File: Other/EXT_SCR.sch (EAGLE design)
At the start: 15 parts, among them IC1 MCP23016-I/SO

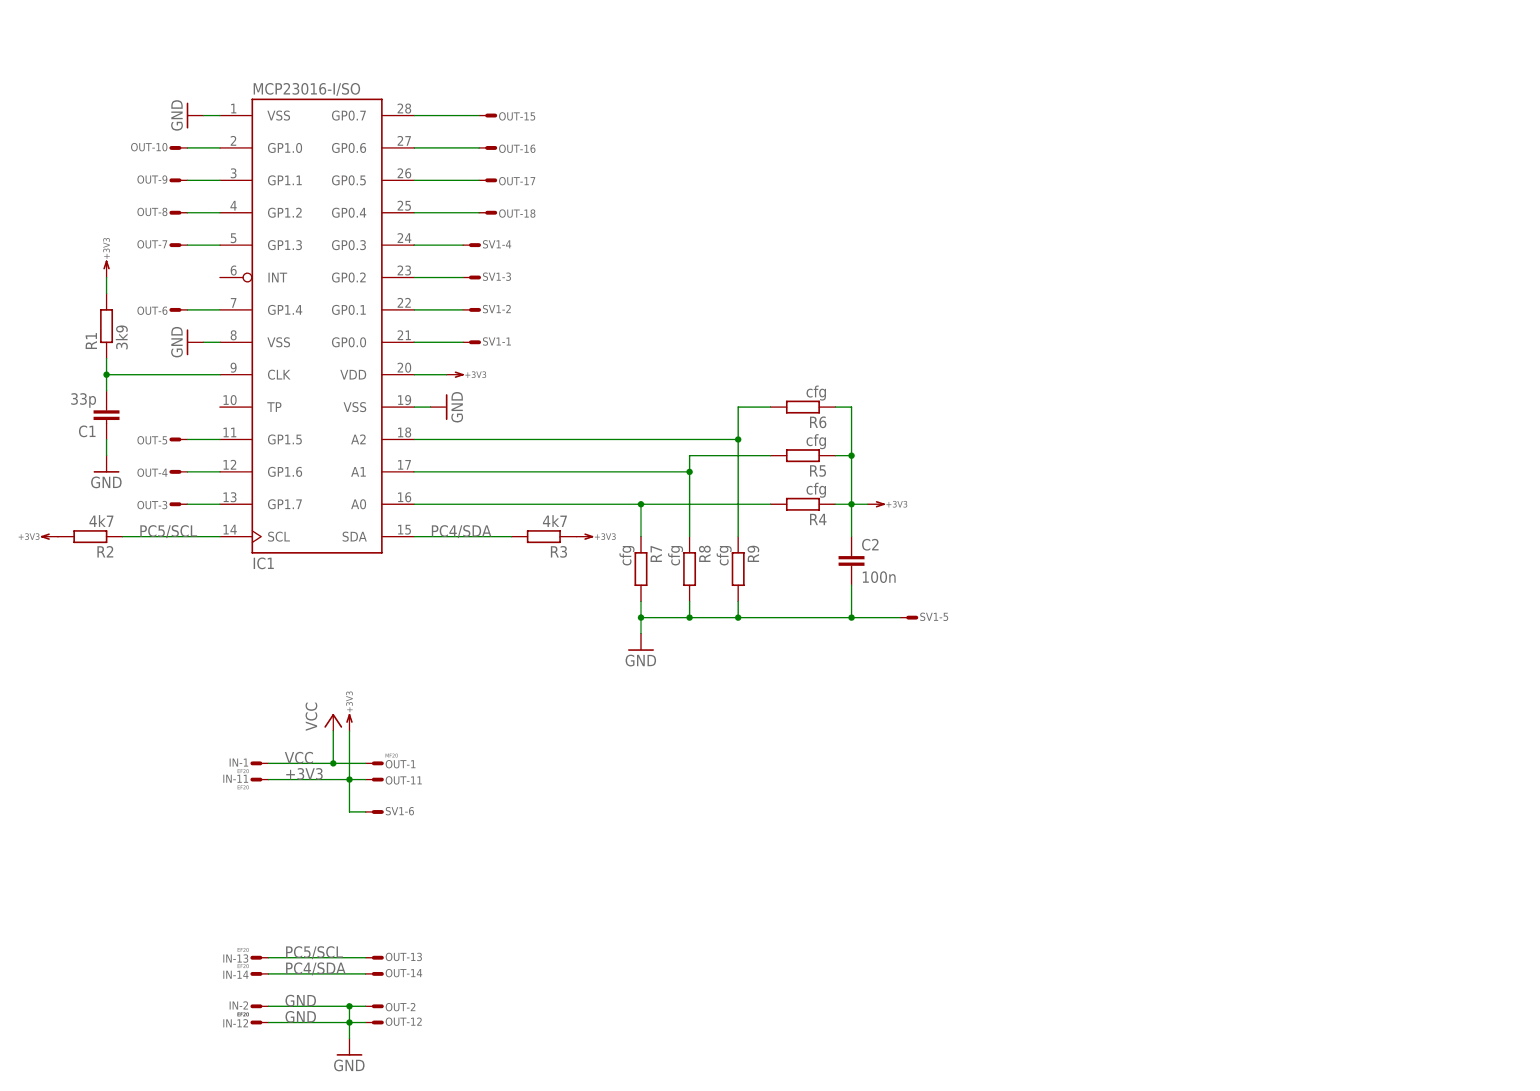
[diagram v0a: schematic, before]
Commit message: Added ...
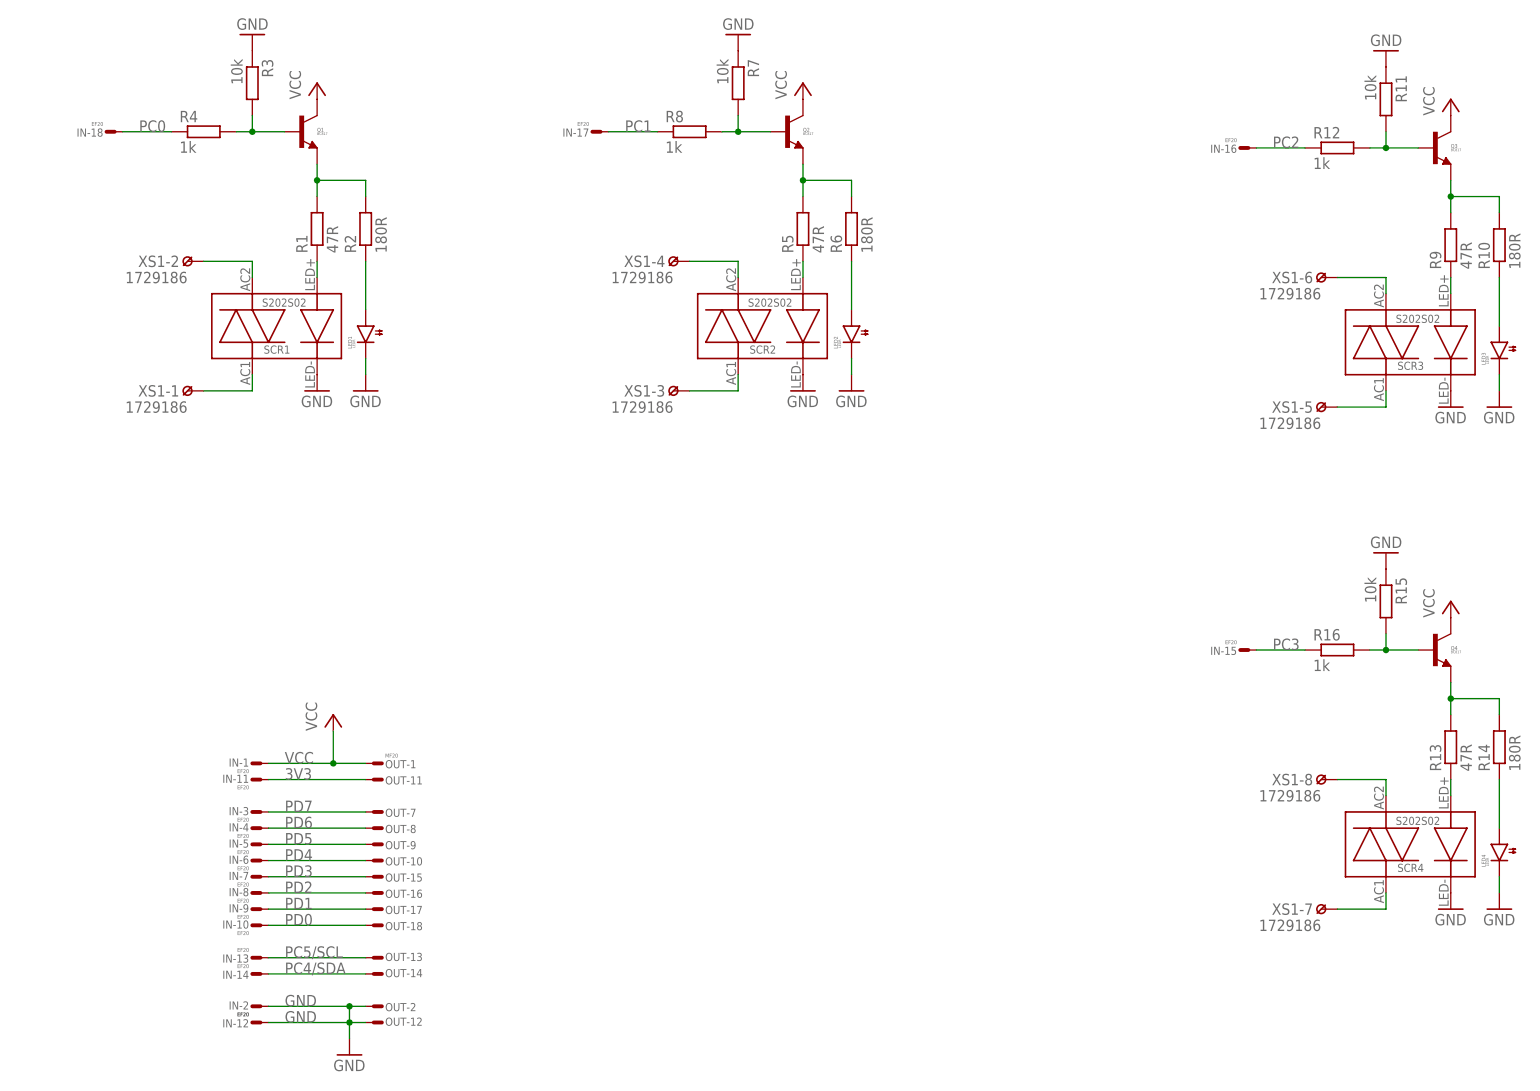
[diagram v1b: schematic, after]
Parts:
- removed C1: 33p, RCL:C0603
- removed C2: 100n, RCL:C0603
- removed IC1: MCP23016-I/SO, ICs:MCP23016-I/SO
- removed SV1: (no value), Conn:ML6ES
- added LED1, LED2, LED3, LED4: LEDR, Optic:LED1206
- added Q1, Q2, Q3, Q4: BC817, Transistor:NPN23
- added R10, R14: 180R, RCL:R0603
- added R11, R15: 10k, RCL:R0603
- added R12, R16: 1k, RCL:R0603
- added R13: 47R, RCL:R0603
- added SCR1, SCR2, SCR3, SCR4: S202S02, Relay_Switch:S202
- added XS1: 1729186, Conn:CON8-SS508
- IN: device Conn:FE20ELSS -> Conn:FE20ELS
- R1: value 3k9 -> 47R
- R2: value 4k7 -> 180R
- R3: value 4k7 -> 10k
- R4, R8: value cfg -> 1k
- R5, R9: value cfg -> 47R
- R6: value cfg -> 180R
- R7: value cfg -> 10k
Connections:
- removed net +3V3: C2.1, IC1.VDD, IN-11.S, OUT-11.S, R1.2, R2.2, R3.1, R4.1, R5.1, R6.1, SV1-6.S
- new net 3V3: IN-11.S, OUT-11.S
- new net N$21: SCR3.AC1, XS1-5.K
- new net N$22: SCR3.AC2, XS1-6.K
- new net N$23: SCR4.AC2, XS1-8.K
- new net N$24: SCR4.AC1, XS1-7.K
- new net PC0: IN-18.S, R4.1
- new net PC1: IN-17.S, R8.1
- new net PC2: IN-16.S, R12.1
- new net PC3: IN-15.S, R16.1
- new net PD0: IN-10.S, OUT-18.S
- new net PD1: IN-9.S, OUT-17.S
- new net PD2: IN-8.S, OUT-16.S
- new net PD3: IN-7.S, OUT-15.S
- new net PD4: IN-6.S, OUT-10.S
- new net PD5: IN-5.S, OUT-9.S
- new net PD6: IN-4.S, OUT-8.S
- new net PD7: IN-3.S, OUT-7.S
- net GND: now also LED1.C, LED2.C, LED3.C, LED4.C, R11.1, R15.1, R3.1, R7.1, SCR1.L-, SCR2.L-, SCR3.L-, SCR4.L-; no longer C1.1, C2.2, IC1.VSS@1, IC1.VSS@19, IC1.VSS@8, R7.2, R8.2, R9.2, SV1-5.S
- net N$1: now also SCR1.L+; no longer C1.2, IC1.CLK
- net N$10: now also LED3.A, R10.1; no longer IC1.A0, R4.2, R7.1
- net N$11: now also Q3.E, R10.2, R9.2; no longer IC1.A1, R5.2, R8.1
- net N$12: now also Q3.B, R11.2, R12.2; no longer IC1.A2, R6.2, R9.1
- net N$13: now also R13.1, SCR4.L+; no longer IC1.GP0.0, SV1-1.S
- net N$14: now also LED4.A, R14.1; no longer IC1.GP0.1, SV1-2.S
- net N$15: now also Q4.E, R13.2, R14.2; no longer IC1.GP0.2, SV1-3.S
- net N$16: now also Q4.B, R15.2, R16.2; no longer IC1.GP0.3, SV1-4.S
- net N$17: now also SCR1.AC1, XS1-1.K; no longer IC1.GP0.4, OUT-18.S
- net N$18: now also SCR1.AC2, XS1-2.K; no longer IC1.GP0.5, OUT-17.S
- net N$19: now also SCR2.AC1, XS1-3.K; no longer IC1.GP0.6, OUT-16.S
- net N$2: now also LED1.A, R2.1; no longer IC1.GP1.4, OUT-6.S
- net N$20: now also SCR2.AC2, XS1-4.K; no longer IC1.GP0.7, OUT-15.S
- net N$3: now also Q1.E, R1.2, R2.2; no longer IC1.GP1.3, OUT-7.S
- net N$4: now also Q1.B, R3.2, R4.2; no longer IC1.GP1.2, OUT-8.S
- net N$5: now also R5.1, SCR2.L+; no longer IC1.GP1.1, OUT-9.S
- net N$6: now also LED2.A, R6.1; no longer IC1.GP1.0, OUT-10.S
- net N$7: now also Q2.E, R5.2, R6.2; no longer IC1.GP1.5, OUT-5.S
- net N$8: now also Q2.B, R7.2, R8.2; no longer IC1.GP1.6, OUT-4.S
- net N$9: now also R9.1, SCR3.L+; no longer IC1.GP1.7, OUT-3.S
- net PC4/SDA: no longer IC1.SDA, R3.2
- net PC5/SCL: no longer IC1.SCL, R2.1
- net VCC: now also Q1.C, Q2.C, Q3.C, Q4.C
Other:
- moved on the sheet: OUT-10, OUT-15, OUT-16, OUT-17, OUT-18, OUT-7, OUT-8, OUT-9, R1, R2, R3, R4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

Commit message: Reorganization
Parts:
- IN: device Conn:FE20ELS -> Conn:FE20ELSS
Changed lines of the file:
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@@
 <?xml version="1.0" encoding="utf-8"?>
 <!DOCTYPE eagle SYSTEM "eagle.dtd">
-<eagle version="6.4">
+<eagle version="6.5.0">
 <drawing>
 <settings>
@@
 <grid distance="0.1" unitdist="inch" unit="inch" style="lines" multiple="1" display="no" altdistance="0.01" altunitdist="inch" altunit="inch"/>
 <layers>
-<layer number="1" name="Top" color="4" fill="1" visible="no" active="no"/>
-<layer number="2" name="Route2" color="1" fill="3" visible="no" active="no"/>
-<layer number="3" name="Route3" color="4" fill="3" visible="no" active="no"/>
-<layer number="4" name="Route4" color="1" fill="4" visible="no" active="no"/>
-<layer number="5" name="Route5" color="4" fill="4" visible="no" active="no"/>
-<layer number="6" name="Route6" color="1" fill="8" visible="no" active="no"/>
-<layer number="7" name="Route7" color="4" fill="8" visible="no" active="no"/>
-<layer number="8" name="Route8" color="1" fill="2" visible="no" active="no"/>
-<layer number="9" name="Route9" color="4" fill="2" visible="no" active="no"/>
-<layer number="10" name="Route10" color="1" fill="7" visible="no" active="no"/>
-<layer number="11" name="Route11" color="4" fill="7" visible="no" active="no"/>
-<layer number="12" name="Route12" color="1" fill="5" visible="no" active="no"/>
-<layer number="13" name="Route13" color="4" fill="5" visible="no" active="no"/>
-<layer number="14" name="Route14" color="1" fill="6" visible="no" active="no"/>
-<layer number="15" name="Route15" color="4" fill="6" visible="no" active="no"/>
-<layer number="16" name="Bottom" color="1" fill="1" visible="no" active="no"/>
-<layer number="17" name="Pads" color="2" fill="1" visible="no" active="no"/>
-<layer number="18" name="Vias" color="2" fill="1" visible="no" active="no"/>
-<layer number="19" name="Unrouted" color="6" fill="1" visible="no" active="no"/>
-<layer number="20" name="Dimension" color="15" fill="1" visible="no" active="no"/>
-<layer number="21" name="tPlace" color="7" fill="1" visible="no" active="no"/>
-<layer number="22" name="bPlace" color="7" fill="1" visible="no" active="no"/>
-<layer number="23" name="tOrigins" color="15" fill="1" visible="no" active="no"/>
-<layer number="24" name="bOrigins" color="15" fill="1" visible="no" active="no"/>
-<layer number="25" name="tNames" color="7" fill="1" visible="no" active="no"/>
-<layer number="26" name="bNames" color="7" fill="1" visible="no" active="no"/>
-<layer number="27" name="tValues" color="7" fill="1" visible="no" active="no"/>
-<layer number="28" name="bValues" color="7" fill="1" visible="no" active="no"/>
+<layer number="1" name="Top" color="4" fill="1" visible="yes" active="no"/>
+<layer number="2" name="Route2" color="1" fill="3" visible="yes" active="no"/>
+<layer number="3" name="Route3" color="4" fill="3" visible="yes" active="no"/>
+<layer number="4" name="Route4" color="1" fill="4" visible="yes" active="no"/>
+<layer number="5" name="Route5" color="4" fill="4" visible="yes" active="no"/>
+<layer number="6" name="Route6" color="1" fill="8" visible="yes" active="no"/>
+<layer number="7" name="Route7" color="4" fill="8" visible="yes" active="no"/>
+<layer number="8" name="Route8" color="1" fill="2" visible="yes" active="no"/>
+<layer number="9" name="Route9" color="4" fill="2" visible="yes" active="no"/>
+<layer number="10" name="Route10" color="1" fill="7" visible="yes" active="no"/>
+<layer number="11" name="Route11" color="4" fill="7" visible="yes" active="no"/>
+<layer number="12" name="Route12" color="1" fill="5" visible="yes" active="no"/>
+<layer number="13" name="Route13" color="4" fill="5" visible="yes" active="no"/>
+<layer number="14" name="Route14" color="1" fill="6" visible="yes" active="no"/>
+<layer number="15" name="Route15" color="4" fill="6" visible="yes" active="no"/>
+<layer number="16" name="Bottom" color="1" fill="1" visible="yes" active="no"/>
+<layer number="17" name="Pads" color="2" fill="1" visible="yes" active="no"/>
+<layer number="18" name="Vias" color="2" fill="1" visible="yes" active="no"/>
+<layer number="19" name="Unrouted" color="6" fill="1" visible="yes" active="no"/>
+<layer number="20" name="Dimension" color="15" fill="1" visible="yes" active="no"/>
+<layer number="21" name="tPlace" color="7" fill="1" visible="yes" active="no"/>
+<layer number="22" name="bPlace" color="7" fill="1" visible="yes" active="no"/>
+<layer number="23" name="tOrigins" color="15" fill="1" visible="yes" active="no"/>
+<layer number="24" name="bOrigins" color="15" fill="1" visible="yes" active="no"/>
+<layer number="25" name="tNames" color="7" fill="1" visible="yes" active="no"/>
+<layer number="26" name="bNames" color="7" fill="1" visible="yes" active="no"/>
+<layer number="27" name="tValues" color="7" fill="1" visible="yes" active="no"/>
+<layer number="28" name="bValues" color="7" fill="1" visible="yes" active="no"/>
 <layer number="29" name="tStop" color="7" fill="3" visible="no" active="no"/>
 <layer number="30" name="bStop" color="7" fill="6" visible="no" active="no"/>
@@
 <layer number="35" name="tGlue" color="7" fill="4" visible="no" active="no"/>
 <layer number="36" name="bGlue" color="7" fill="5" visible="no" active="no"/>
-<layer number="37" name="tTest" color="7" fill="1" visible="no" active="no"/>
-<layer number="38" name="bTest" color="7" fill="1" visible="no" active="no"/>
+<layer number="37" name="tTest" color="7" fill="1" visible="yes" active="no"/>
+<layer number="38" name="bTest" color="7" fill="1" visible="yes" active="no"/>
 <layer number="39" name="tKeepout" color="4" fill="11" visible="no" active="no"/>
 <layer number="40" name="bKeepout" color="1" fill="11" visible="no" active="no"/>
@@
 <layer number="44" name="Drills" color="7" fill="1" visible="no" active="no"/>
 <layer number="45" name="Holes" color="7" fill="1" visible="no" active="no"/>
-<layer number="46" name="Milling" color="3" fill="1" visible="no" active="no"/>
-<layer number="47" name="Measures" color="7" fill="1" visible="no" active="no"/>
-<layer number="48" name="Document" color="7" fill="1" visible="no" active="no"/>
-<layer number="49" name="Reference" color="7" fill="1" visible="no" active="no"/>
-<layer number="50" name="dxf" color="7" fill="1" visible="no" active="no"/>
-<layer number="51" name="tDocu" color="7" fill="1" visible="no" active="no"/>
-<layer number="52" name="bDocu" color="7" fill="1" visible="no" active="no"/>
-<layer number="53" name="tGND_GNDA" color="7" fill="1" visible="no" active="no"/>
-<layer number="54" name="bGND_GNDA" color="7" fill="1" visible="no" active="no"/>
-<layer number="56" name="wert" color="7" fill="1" visible="no" active="no"/>
+<layer number="46" name="Milling" color="3" fill="1" visible="yes" active="no"/>
+<layer number="47" name="Measures" color="7" fill="1" visible="yes" active="no"/>
+<layer number="48" name="Document" color="7" fill="1" visible="yes" active="no"/>
+<layer number="49" name="Reference" color="7" fill="1" visible="yes" active="no"/>
+<layer number="50" name="dxf" color="7" fill="1" visible="yes" active="no"/>
+<layer number="51" name="tDocu" color="7" fill="1" visible="yes" active="no"/>
+<layer number="52" name="bDocu" color="7" fill="1" visible="yes" active="no"/>
+<layer number="53" name="tGND_GNDA" color="7" fill="1" visible="yes" active="no"/>
+<layer number="54" name="bGND_GNDA" color="7" fill="1" visible="yes" active="no"/>
+<layer number="56" name="wert" color="7" fill="1" visible="yes" active="no"/>
 <layer number="91" name="Nets" color="2" fill="1" visible="yes" active="yes"/>
 <layer number="92" name="Busses" color="1" fill="1" visible="yes" active="yes"/>
@@
 <part name="FRAME1" library="Frames" deviceset="A4L-LOC" device="" value="FR1"/>
 <part name="OUT" library="Conn" deviceset="ML20?E" device="LS" value="MF20"/>
-<part name="IN" library="Conn" deviceset="FE20E" device="LS" value="EF20"/>
+<part name="IN" library="Conn" deviceset="FE20E" device="LSS" value="EF20"/>
 <part name="GND1" library="supply1" deviceset="GND" device=""/>
 <part name="P+7" library="supply1" deviceset="VCC" device=""/>
